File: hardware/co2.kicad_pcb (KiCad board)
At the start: 2 copper layers, 60 x 65 mm, 31 parts, among them P1 CON-SENSOR, U1 M24C64, U2 FAN4860, U3 TLV271, U4 K30, U5 DRILL, U6 DRILL, U7 DRILL, U8 DRILL

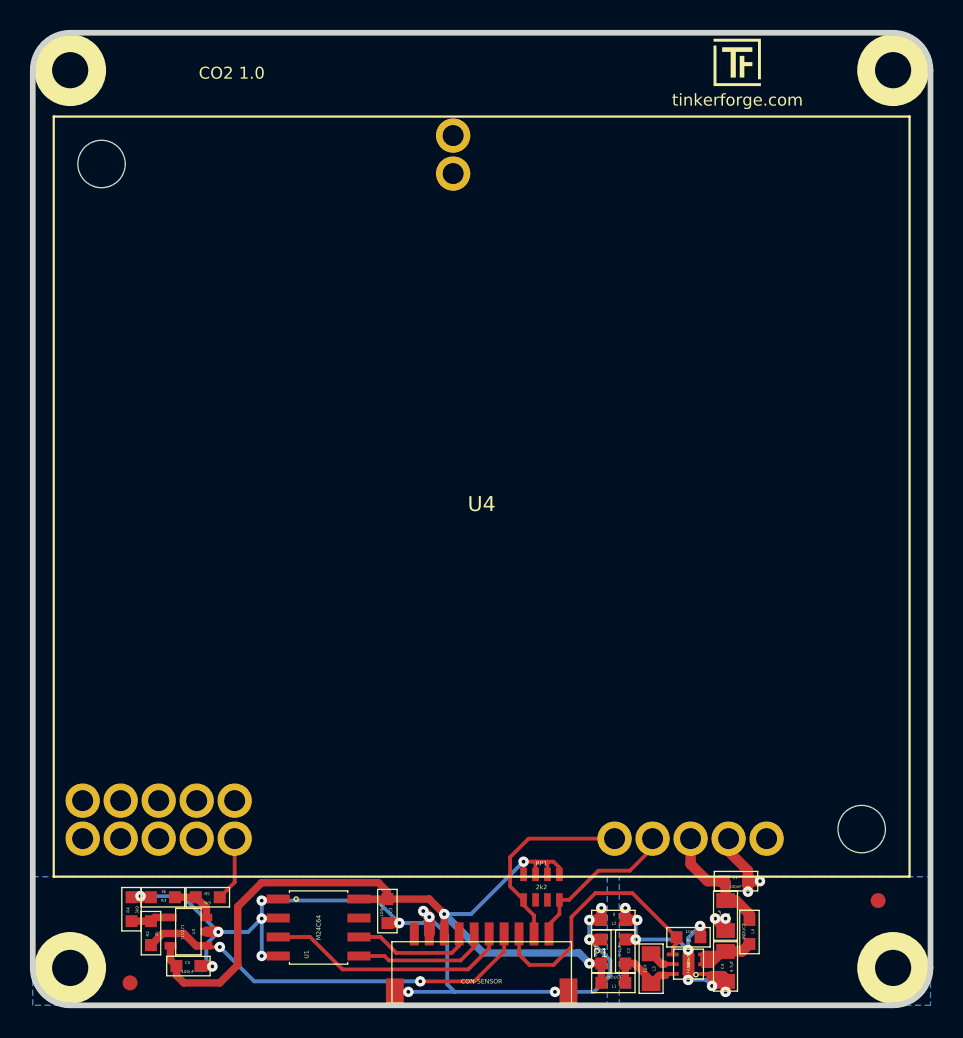
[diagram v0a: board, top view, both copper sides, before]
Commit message: Add 3d information (final)
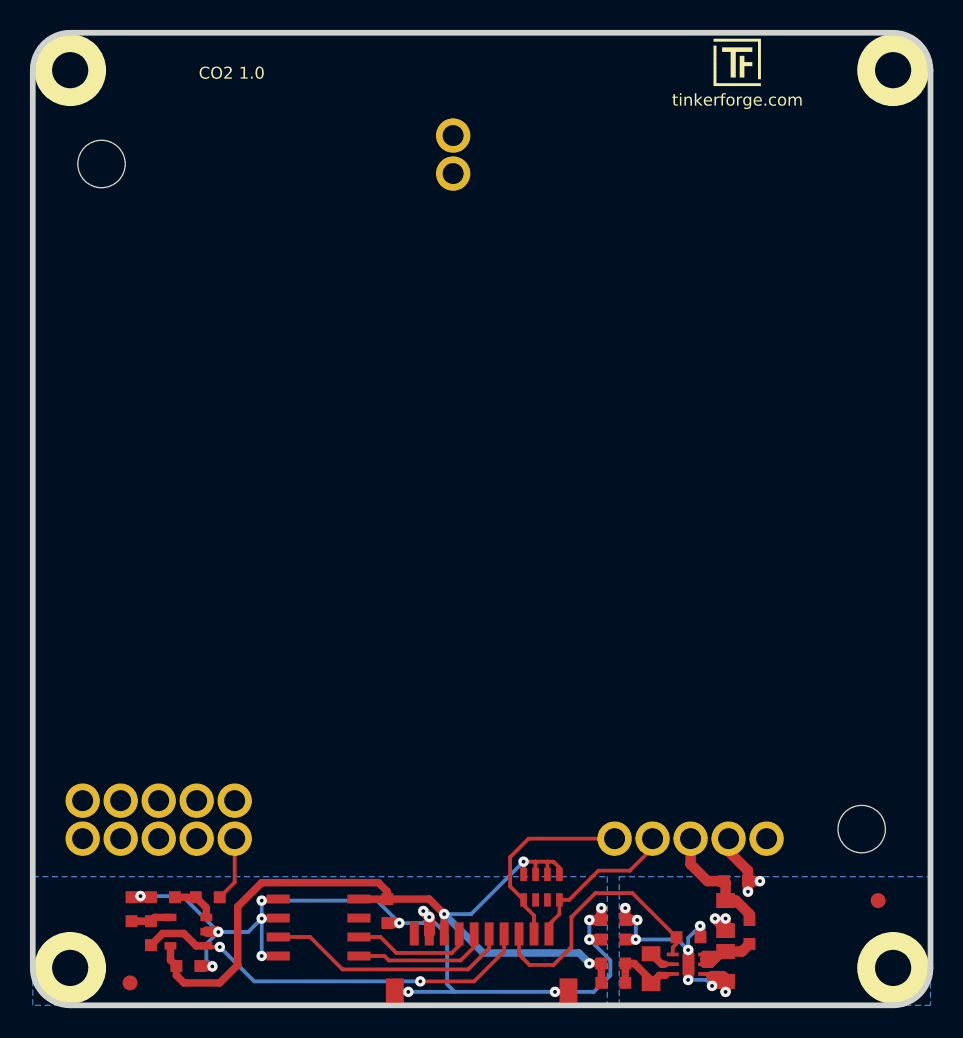
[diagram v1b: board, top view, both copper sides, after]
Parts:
- C1, C2, C3, C5, C7, L1, L2, L4: footprint kicad-libraries:0603 -> kicad-libraries:C0603
- C4, C6, L3: footprint kicad-libraries:0805 -> kicad-libraries:C0805
- R1, R2, R3, R4, R5: footprint kicad-libraries:0603 -> kicad-libraries:R0603
- VAL: footprint kicad-libraries:WEEE_7mm_back -> kicad-libraries:WEEE_7mm
- turned VAL to 180 degrees
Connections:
- P1 pad 1: (no net) -> Net-(P1-Pad1)
- RP1 pad 6: (no net) -> Net-(RP1-Pad6)
- RP1 pad 7: (no net) -> Net-(RP1-Pad7)
- U1 pad 7: (no net) -> Net-(U1-Pad7)
- U4 pad 1: (no net) -> Net-(U4-Pad1)
- U4 pad 10: (no net) -> Net-(U4-Pad10)
- U4 pad 11: (no net) -> Net-(U4-Pad11)
- U4 pad 12: (no net) -> Net-(U4-Pad12)
- U4 pad 13: (no net) -> Net-(U4-Pad13)
- U4 pad 14: (no net) -> Net-(U4-Pad14)
- U4 pad 6: (no net) -> Net-(U4-Pad6)
- U4 pad 7: (no net) -> Net-(U4-Pad7)
- U4 pad 8: (no net) -> Net-(U4-Pad8)
- U4 pad 9: (no net) -> Net-(U4-Pad9)
